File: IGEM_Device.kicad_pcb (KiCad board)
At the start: 2 copper layers, 50.2 x 47 mm, 28 parts, among them J1 67997-410HLF, J2 Electrode_Conn, J3 Batt_Conn, SW1 Power_Switch, U1 SaBLE-X-R2, U2 TC1014-2.85VCT713, U3 LMP91000SD_NOPB, U4 LM334MX_NOPB, U5 TPS79718QDCKRQ1, U6 G-NIMO-003

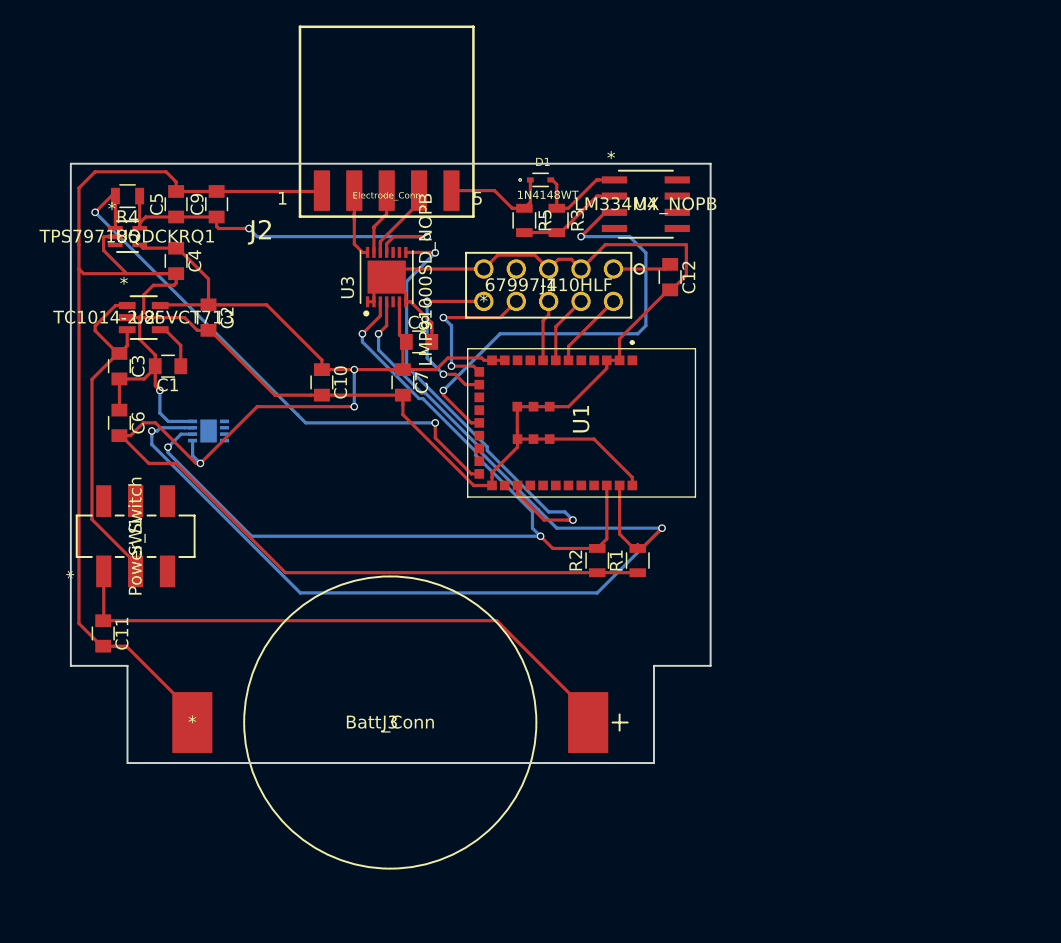
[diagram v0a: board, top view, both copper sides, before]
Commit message: Minor fixes
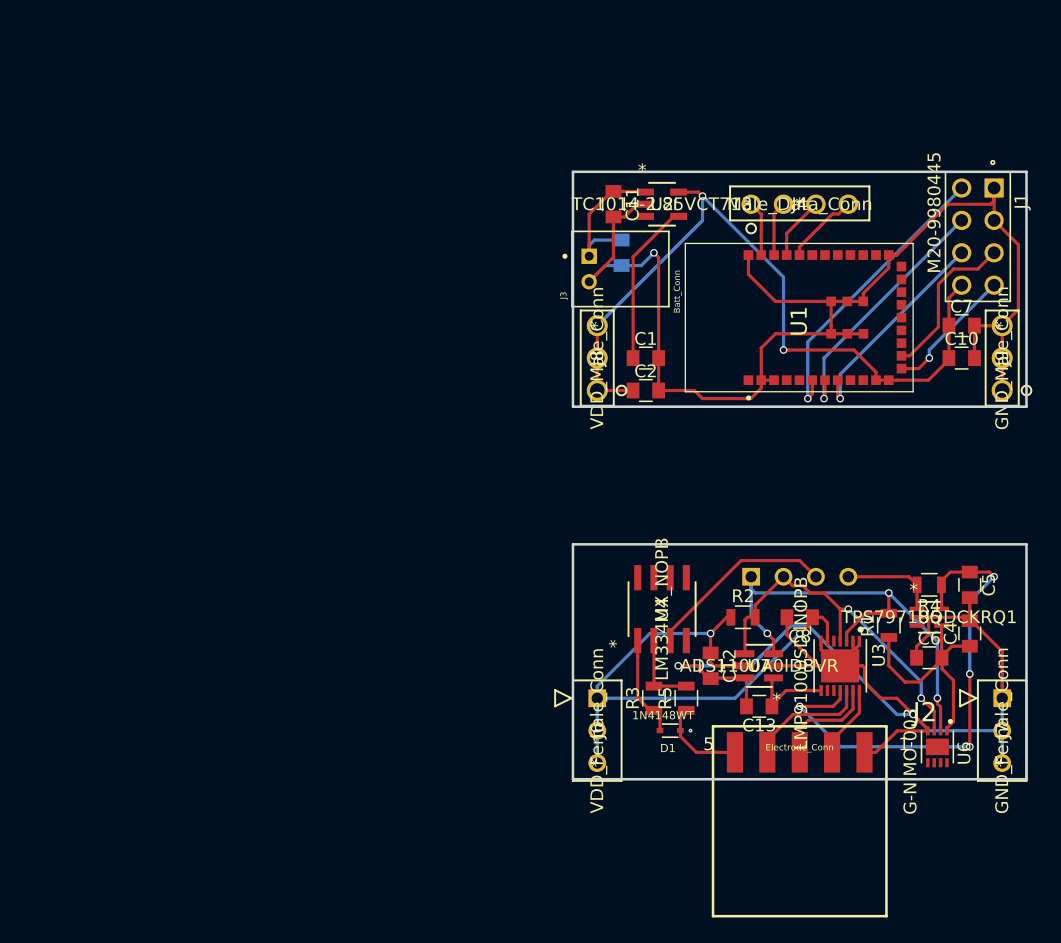
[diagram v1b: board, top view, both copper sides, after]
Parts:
- removed C9: 0.1u, Capacitors_SMD:C_0805
- removed SW1: Power_Switch, footprints5:JS202011SCQN
- added C13: 100p, Capacitors_SMD:C_0805, F.Cu at (154.3, 93.3)
- added J4: Male_Data_Conn, HTSW10407GS:HTSW-104-07-G-S, F.Cu at (157.5, 54.0)
- added J5: Female_Data_Conn, 55342372:5-534237-2, B.Cu at (161.3, 83.2)
- added J6: VDD_Female_Conn, 55342371:5-534237-1, F.Cu at (141.6, 97.8)
- added J7: GND_Female_Conn, 55342371:5-534237-1, F.Cu at (173.4, 97.8)
- added J8: VDD_Male_Conn, 51462803:5-146280-3, F.Cu at (141.6, 63.5)
- added J9: GND_Male_Conn, 51462803:5-146280-3, F.Cu at (173.4, 63.5)
- added U7: ADS1100A0IDBVR, ADS1100A0TDBVR:ADS1100A0IDBVR, F.Cu at (154.3, 90.2)
- C3: moved to B.Cu
- D1: footprint SODFL1608X70N -> 1N4148WT:SODFL1608X70N
- J1: value 67997-410HLF -> M20-9980445; footprint footprints3:67997-410HLF -> M20-9980445:HDRV8W64P254_2X4_1016X508X910P
- J3: footprint footprints6:796136-1 -> S2B-PH-K-S_LF__SN_:JST_S2B-PH-K-S(LF)(SN)
- U6: moved to F.Cu
- moved R4 69.9 mm to (167.6, 83.8)
- moved U5 69.6 mm to (167.6, 86.4)
- moved C5 69.0 mm to (170.8, 83.8), turned to 270 degrees
- moved C4 68.7 mm to (170.8, 87.6), turned to 90 degrees
- moved C6 66.1 mm to (167.6, 89.5), turned to 0 degrees
- moved J2 63.5 mm to (157.5, 102.2), turned to 180 degrees
- moved U6 62.3 mm to (168.3, 96.5), turned to 270 degrees
- moved C11 52.3 mm to (142.9, 54.0)
- moved C10 50.2 mm to (170.2, 66.0), turned to 0 degrees
- moved J3 47.3 mm to (141.0, 59.1), turned to 90 degrees
- moved U3 46.8 mm to (160.7, 90.2), turned to 270 degrees
- moved D1 44.4 mm to (147.3, 95.2), turned to 180 degrees
- moved C7 44.0 mm to (170.2, 63.5), turned to 0 degrees
- moved U2 41.6 mm to (146.7, 54.0)
- moved J1 41.0 mm to (172.7, 52.7), turned to 270 degrees
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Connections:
- C12 pad 1: +3V3 -> +2V85
- C3 pad 1: Net-(C3-Pad1) -> +BATT
- J1 pad 1: +3V3 -> GND
- J1 pad 2: GND -> /RESET
- J1 pad 4: Net-(J1-Pad4) -> /JTAG_TCXC
- J1 pad 5: GND -> /JTAG_TDI
- J1 pad 6: /RESET -> /JTAG_TMSC
- J1 pad 7: /JTAG_TCXC -> /JTAG_TDO
- J1 pad 8: /JTAG_TMSC -> +2V85
- R1 pad 2: /EXT_TEMP_SDA -> /SCL
- R2 pad 2: /EXT_TEMP_SCL -> /SDA
- U1 pad 17: /IP_CONTROL -> Net-(U1-Pad17)
- U1 pad 21: /POWER_GOOD -> Net-(U1-Pad21)
- U1 pad 24: /TEMP_OUT -> Net-(U1-Pad24)
- U1 pad 29: Net-(U1-Pad29) -> /POWER_GOOD
- U1 pad 30: Net-(U1-Pad30) -> /IP_CONTROL
- U1 pad 31: /EXT_TEMP_SCL -> /SDA
- U1 pad 32: /EXT_TEMP_SDA -> /SCL
- U2 pad 1: Net-(C3-Pad1) -> +BATT
- U2 pad 3: Net-(C3-Pad1) -> +BATT
- U3 pad 3: /EXT_TEMP_SCL -> /SCL
- U3 pad 4: /EXT_TEMP_SDA -> /SDA
- U3 pad 8: /TEMP_OUT -> /LMP91000_VOUT
- U6 pad 2: /EXT_TEMP_SCL -> /SCL
- U6 pad 3: /EXT_TEMP_SDA -> /SDA
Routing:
- net /EXT_TEMP_SDA: track 92.1 -> 0.00 mm, vias 3 -> 0
- net /EXT_TEMP_SCL: track 69.7 -> 0.00 mm, vias 3 -> 0
- net /SCL: track 0.00 -> 42.2 mm, vias 0 -> 3
- net /TEMP_OUT: track 36.2 -> 0.00 mm, vias 2 -> 0
- net +BATT: track 45.7 -> 12.0 mm
- net /SDA: track 0.00 -> 32.9 mm, vias 0 -> 2
- net /POWER_GOOD: track 44.0 -> 13.4 mm, vias 2 -> 0
- net Net-(C3-Pad1): track 27.7 -> 0.00 mm
- net GND: track 213.5 -> 194.1 mm, vias 1 -> 3
- net /IP_CONTROL: track 37.5 -> 19.9 mm, vias 2 -> 0
- net /RESET: track 6.08 -> 23.1 mm, vias 0 -> 1
- net /JTAG_TCXC: track 5.44 -> 19.9 mm, vias 0 -> 1
- net /JTAG_TMSC: track 4.80 -> 16.9 mm, vias 0 -> 1
- net Net-(C1-Pad1): track 3.75 -> 12.8 mm
- net +1V8: track 30.8 -> 39.6 mm, vias 2 -> 4
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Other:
- board size 50.2 x 47 mm -> 35.6 x 47.6 mm
